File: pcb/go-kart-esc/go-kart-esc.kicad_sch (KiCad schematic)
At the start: 0 parts

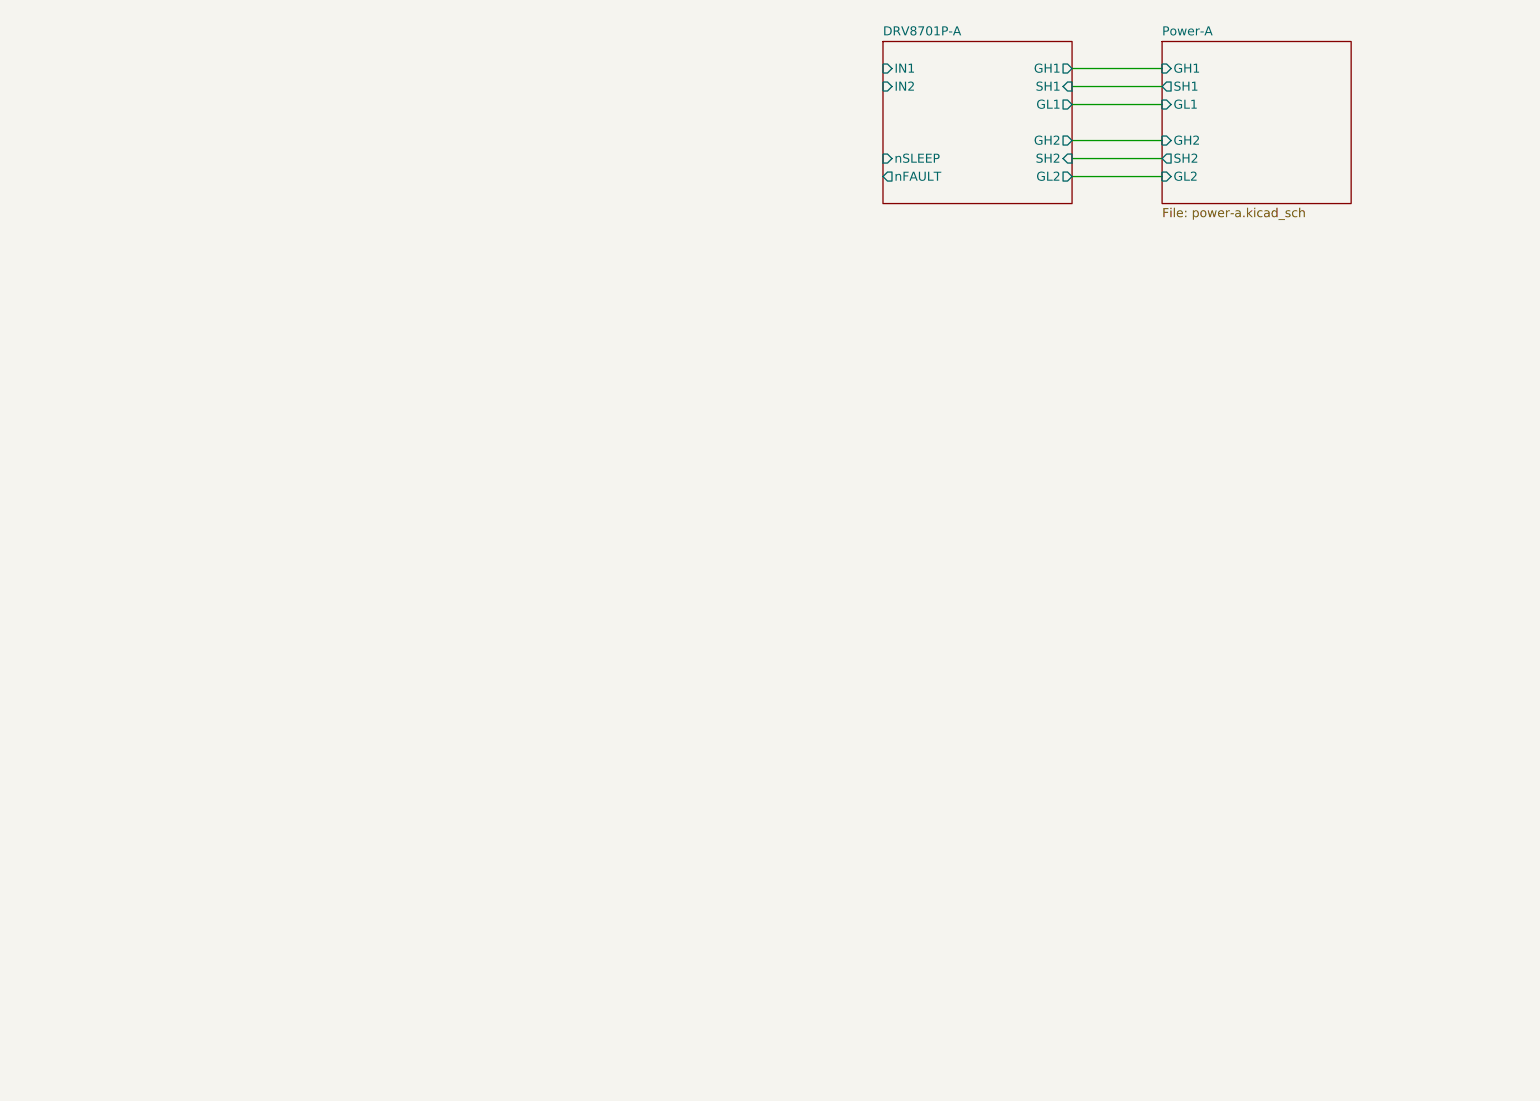
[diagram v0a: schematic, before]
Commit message: Poggers
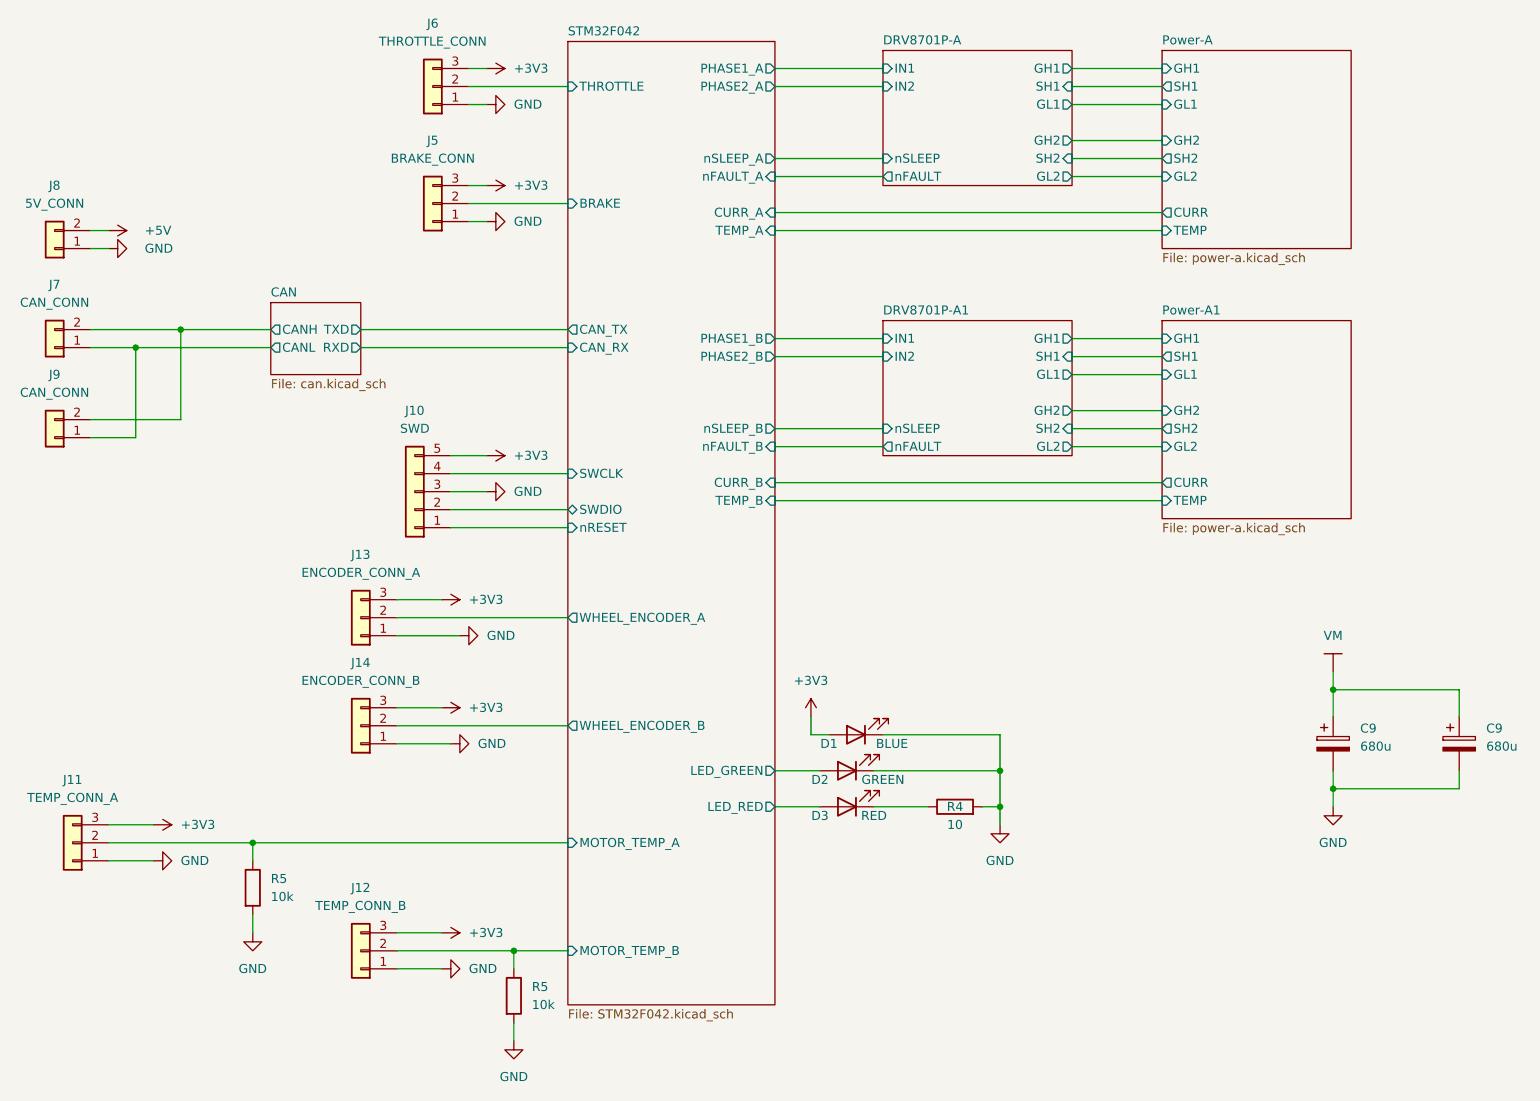
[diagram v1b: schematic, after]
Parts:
- added C9 (x2): 680u, symbol Device:C_Polarized
- added D1: BLUE, symbol Device:LED
- added D2: GREEN, symbol Device:LED
- added D3: RED, symbol Device:LED
- added J10: SWD, symbol Connector_Generic:Conn_01x05
- added J11: TEMP_CONN_A, Connector_JST:JST_PH_S3B-PH-K_1x03_P2.00mm_Horizontal, symbol Connector_Generic:Conn_01x03
- added J12: TEMP_CONN_B, Connector_JST:JST_PH_S3B-PH-K_1x03_P2.00mm_Horizontal, symbol Connector_Generic:Conn_01x03
- added J13: ENCODER_CONN_A, Connector_JST:JST_PH_S3B-PH-K_1x03_P2.00mm_Horizontal, symbol Connector_Generic:Conn_01x03
- added J14: ENCODER_CONN_B, Connector_JST:JST_PH_S3B-PH-K_1x03_P2.00mm_Horizontal, symbol Connector_Generic:Conn_01x03
- added J5: BRAKE_CONN, Connector_JST:JST_PH_S3B-PH-K_1x03_P2.00mm_Horizontal, symbol Connector_Generic:Conn_01x03
- added J6: THROTTLE_CONN, Connector_JST:JST_PH_S3B-PH-K_1x03_P2.00mm_Horizontal, symbol Connector_Generic:Conn_01x03
- added J7, J9: CAN_CONN, symbol Connector_Generic:Conn_01x02
- added J8: 5V_CONN, symbol Connector_Generic:Conn_01x02
- added R4: 10, symbol Device:R
- added R5 (x2): 10k, symbol Device:R
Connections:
- new net: C9.1, C9.1
- new net: D3.1 (K), R4.1
- new net +3V3: D1.2 (A), J10.5 (Pin_5), J11.3 (Pin_3), J12.3 (Pin_3), J13.3 (Pin_3), J14.3 (Pin_3), J5.3 (Pin_3), J6.3 (Pin_3)
- new net +5V: J8.2 (Pin_2)
- new net CAN/CANH: J7.2 (Pin_2), J9.2 (Pin_2)
- new net CAN/CANL: J7.1 (Pin_1), J9.1 (Pin_1)
- new net GND: C9.2, C9.2, D1.1 (K), D2.1 (K), J10.3 (Pin_3), J11.1 (Pin_1), J12.1 (Pin_1), J13.1 (Pin_1), J14.1 (Pin_1), J5.1 (Pin_1), J6.1 (Pin_1), J8.1 (Pin_1), R4.2, R5.2, R5.2
- new net STM32F042/BRAKE: J5.2 (Pin_2)
- new net STM32F042/LED_GREEN: D2.2 (A)
- new net STM32F042/LED_RED: D3.2 (A)
- new net STM32F042/MOTOR_TEMP_A: J11.2 (Pin_2), R5.1
- new net STM32F042/MOTOR_TEMP_B: J12.2 (Pin_2), R5.1
- new net STM32F042/SWCLK: J10.4 (Pin_4)
- new net STM32F042/SWDIO: J10.2 (Pin_2)
- new net STM32F042/THROTTLE: J6.2 (Pin_2)
- new net STM32F042/WHEEL_ENCODER_A: J13.2 (Pin_2)
- new net STM32F042/WHEEL_ENCODER_B: J14.2 (Pin_2)
- new net STM32F042/nRESET: J10.1 (Pin_1)
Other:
- added sheet CAN (can.kicad_sch)
- added sheet DRV8701P-A1 (DRV8701P-A.kicad_sch)
- added sheet Power-A1 (power-a.kicad_sch)
- added sheet STM32F042 (STM32F042.kicad_sch)
- sheet Power-A ports: added CURR, TEMP; removed none
